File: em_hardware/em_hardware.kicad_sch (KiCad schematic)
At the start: 7 parts, among them SW1 SW_Push, SW2 SW_Push, U1 ESP32-WROOM-32

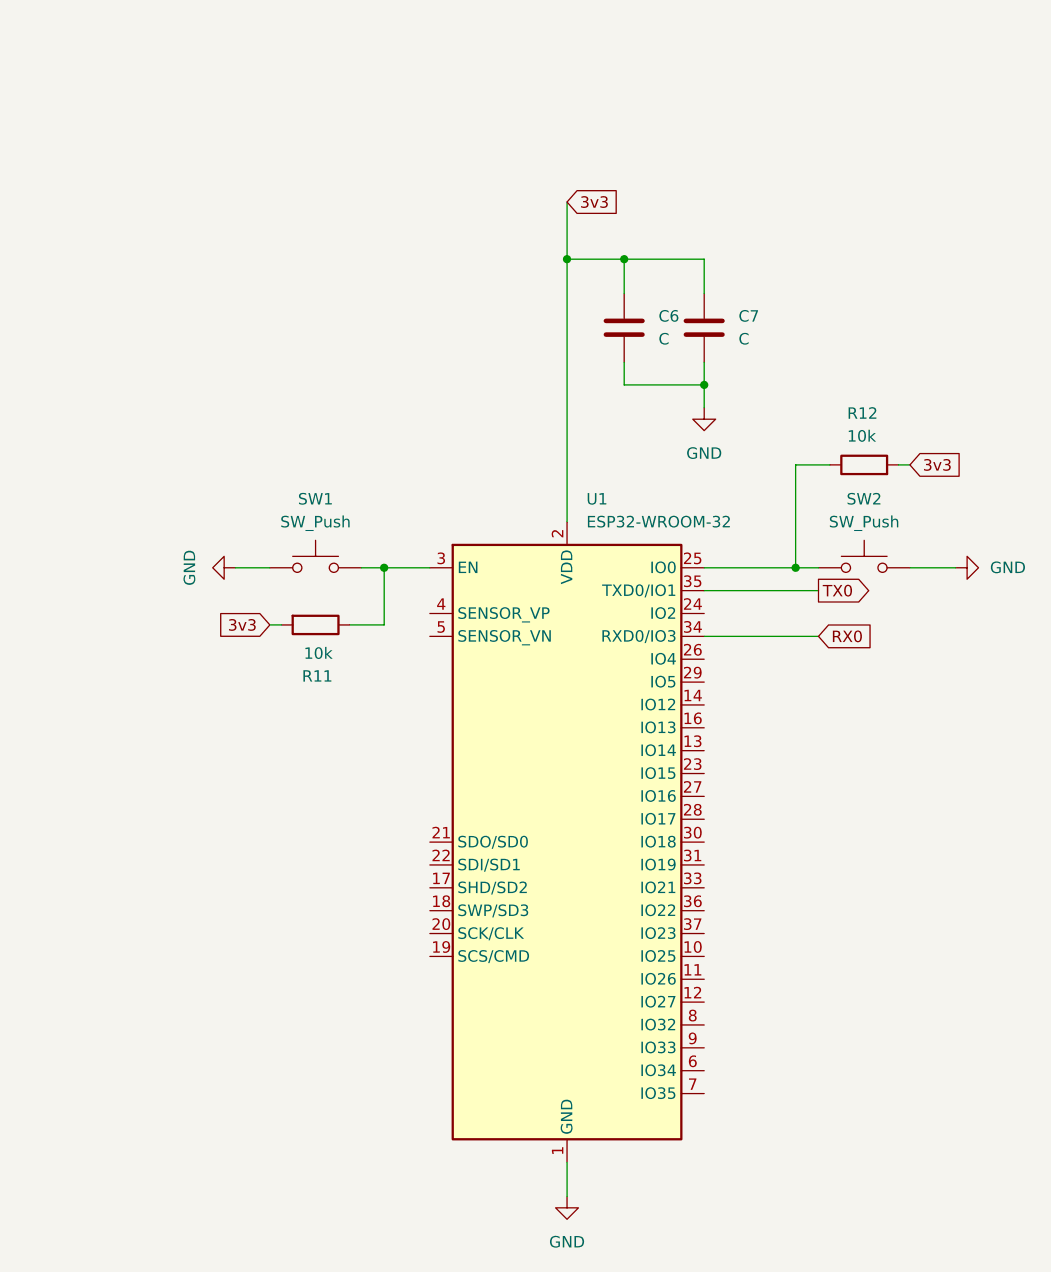
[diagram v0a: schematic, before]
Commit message: done the power
sensors next
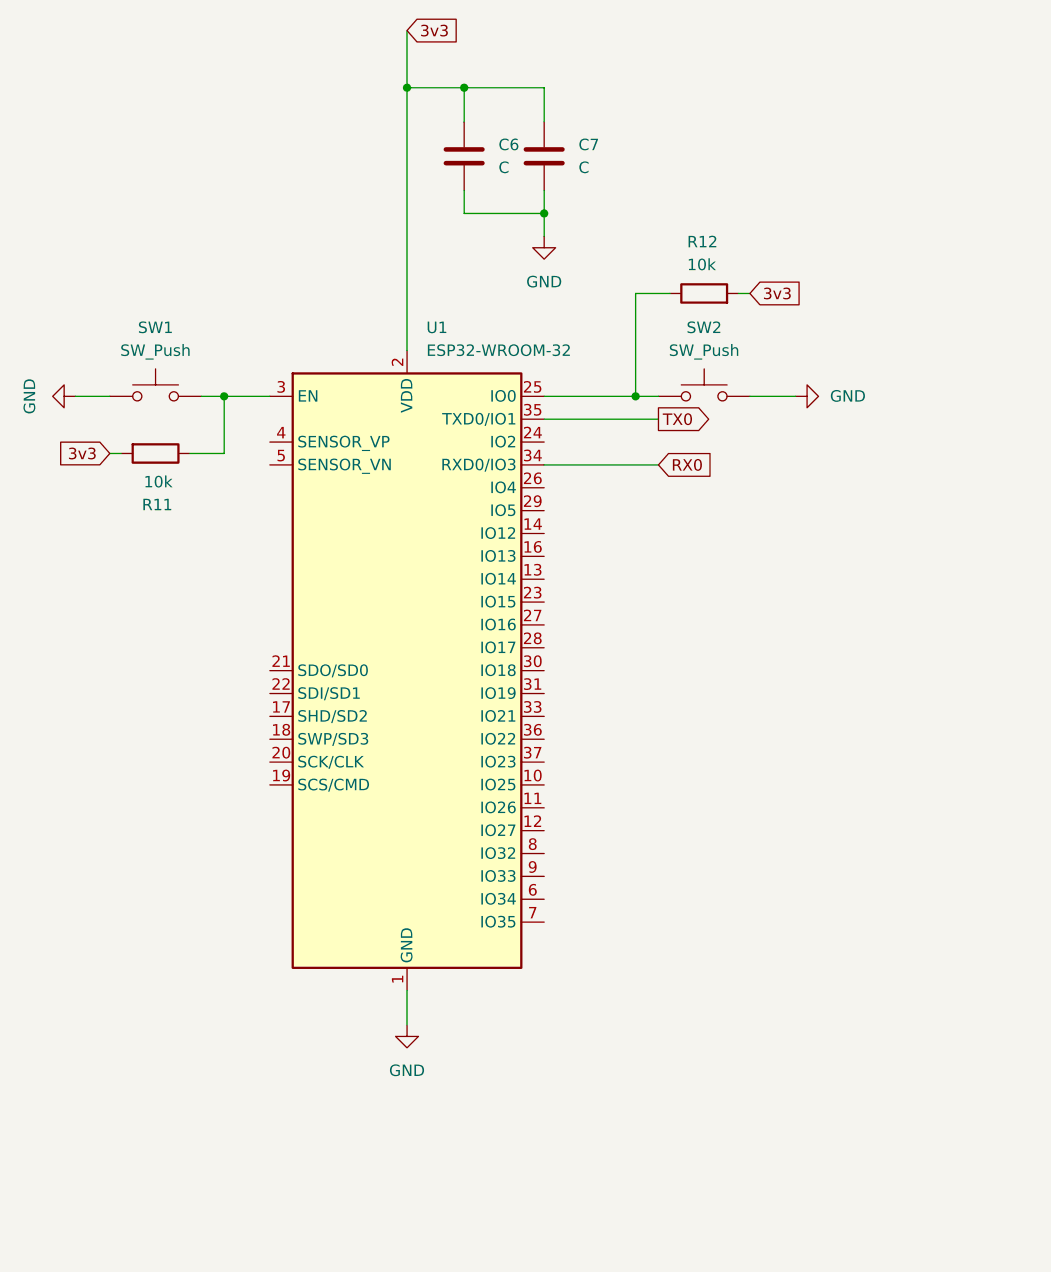
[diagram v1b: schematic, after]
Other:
- moved on the sheet: C6, C7, R11, R12, SW1, SW2, U1
